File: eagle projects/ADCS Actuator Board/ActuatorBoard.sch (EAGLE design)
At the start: 281 parts, among them J19 TE_1-84953-1, J20 TE_1-84953-1, J21 TE_1-84953-1, U1 TVS991, U10 DRV10970_MOTOR_DRIVERDRV10970, U12 DRV10970_MOTOR_DRIVERDRV10970, U13 ADS7841E_2K5, U15 TLV9051IDCKR, U19 TLV9051IDCKR, U2 ADS7841E_2K5, U21 TLV9051IDCKR, U23 TLV9051IDCKR, U24 TLV9051IDCKR, U25 ADS7841E_2K5, U26 TLV9051IDCKR, U27 ADS7841E_2K5, U28 TLV9051IDCKR, U29 TLV9051IDCKR, U3 ADS7841E_2K5, U30 TLV9051IDCKR, U31 TLV9051IDCKR, U32 TLV9051IDCKR, U35 BD6210F-E2, U39 BD6210F-E2, U4 ADS7841E_2K5, U5 TVS991, U6 TLV9051IDCKR, U7 DRV10970_MOTOR_DRIVERDRV10970, U8 TVS991, U9 BD6210F-E2

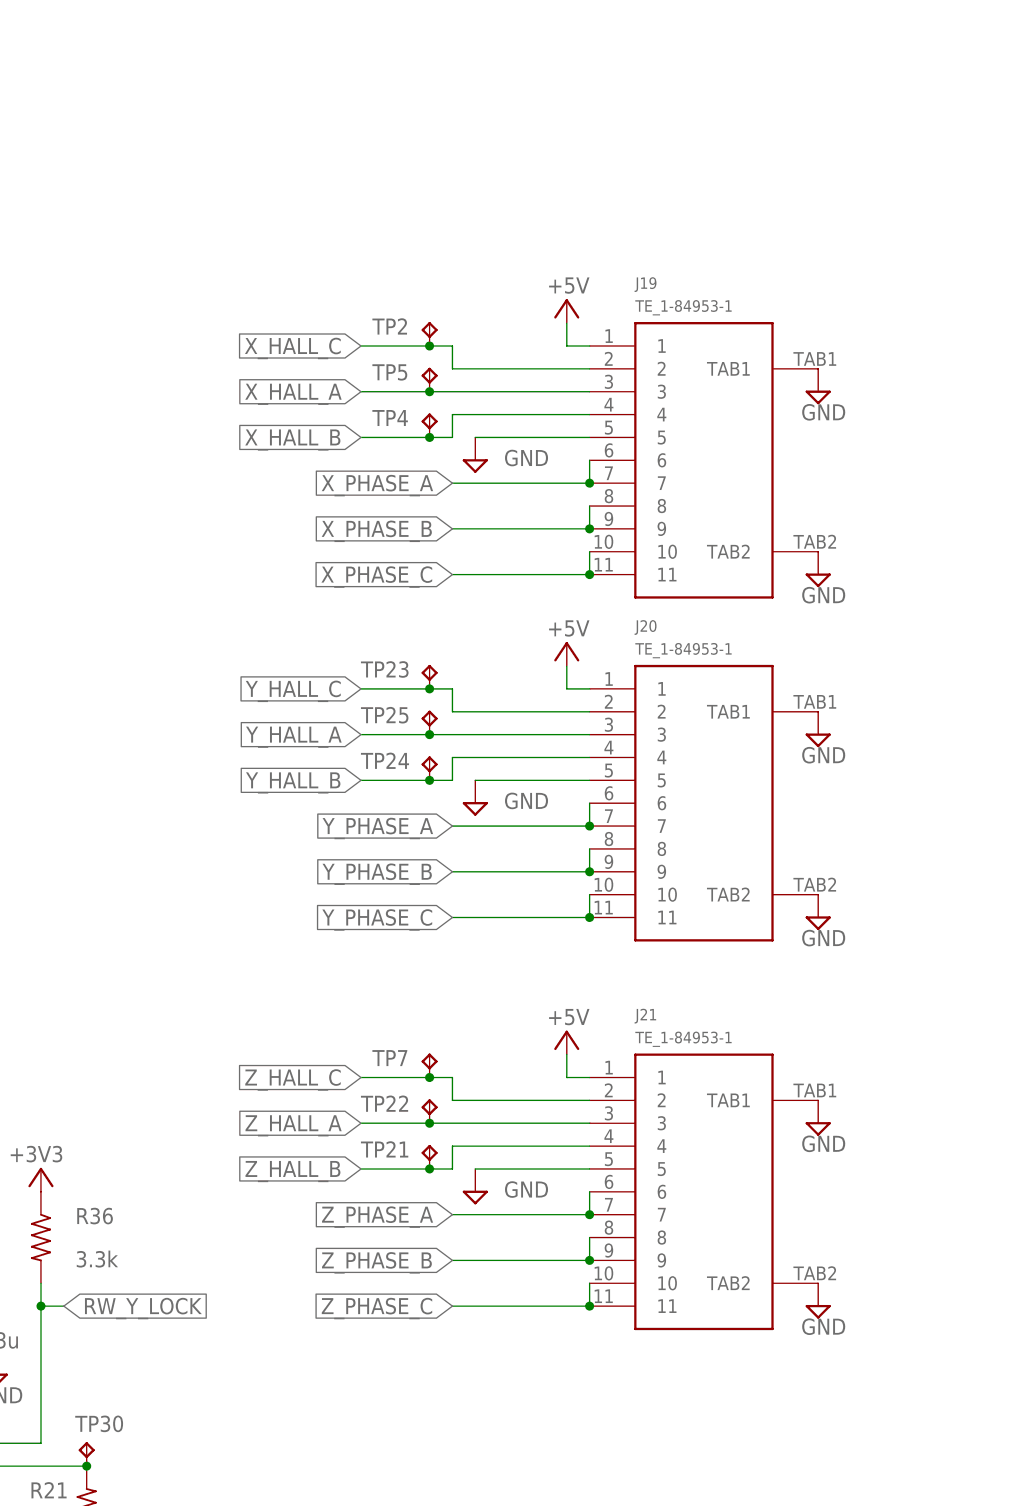
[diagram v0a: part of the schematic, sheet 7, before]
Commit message: DONE THIS MFER
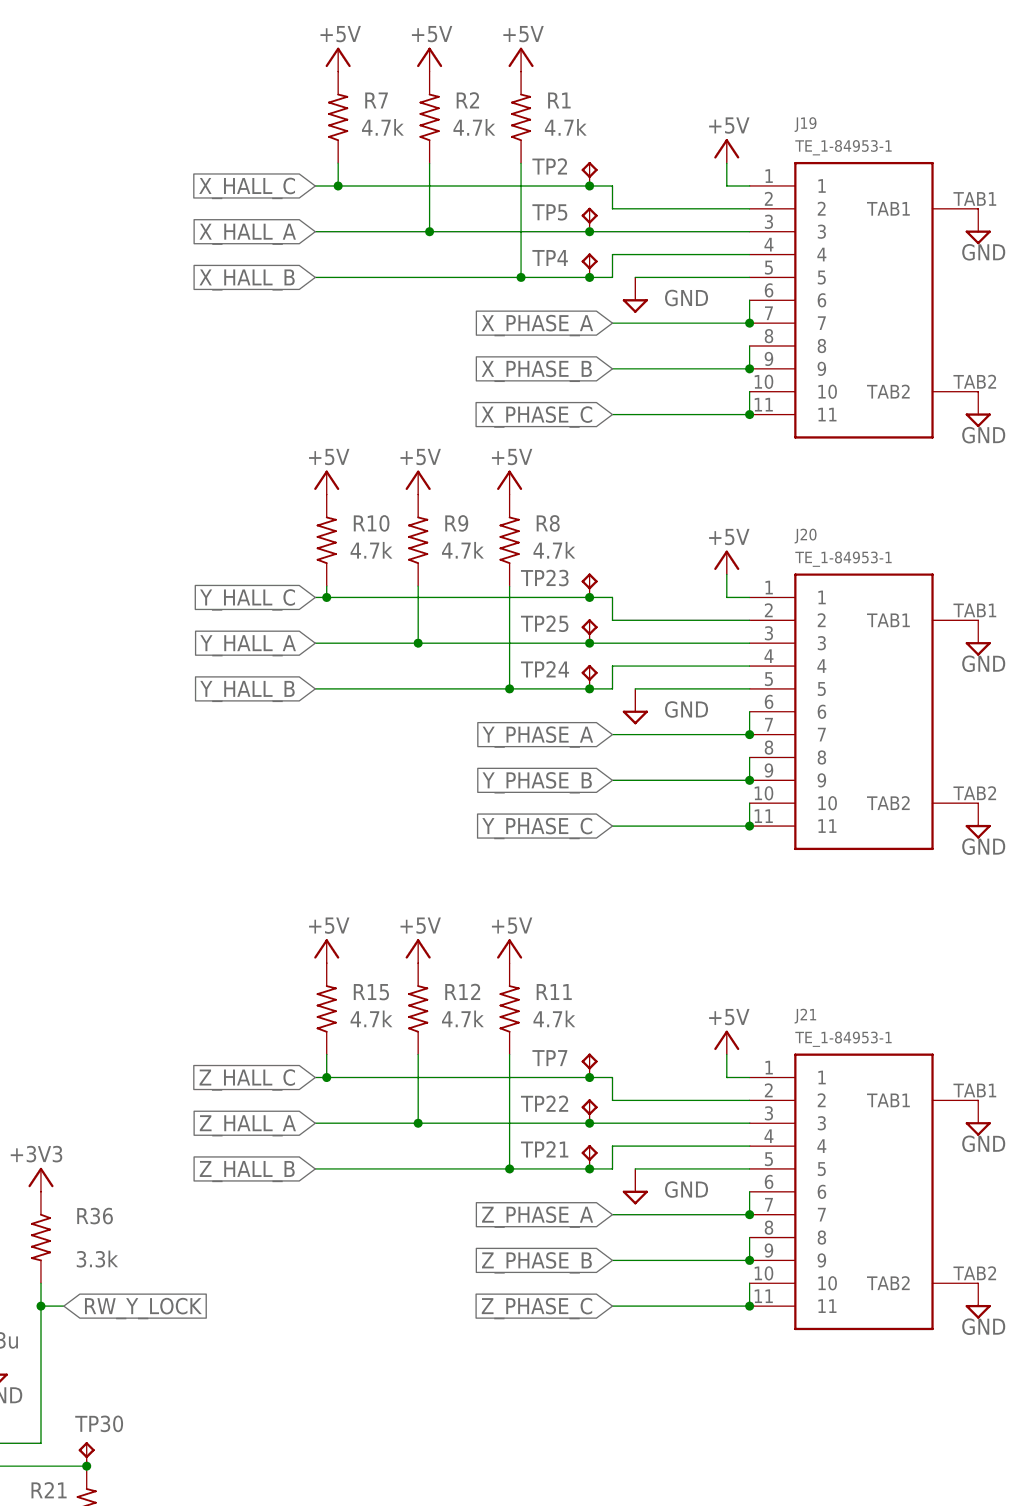
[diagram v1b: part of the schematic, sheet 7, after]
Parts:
- added R1, R10, R11, R12, R15, R2, R7, R8, R9: 4.7k, rcl:R-US_R0402
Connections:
- net +5V: now also R1.2, R10.2, R11.2, R12.2, R15.2, R2.2, R7.2, R8.2, R9.2
- net X_HALL_A: now also R2.1
- net X_HALL_B: now also R1.1
- net X_HALL_C: now also R7.1
- net Y_HALL_A: now also R9.1
- net Y_HALL_B: now also R8.1
- net Y_HALL_C: now also R10.1
- net Z_HALL_A: now also R12.1
- net Z_HALL_B: now also R11.1
- net Z_HALL_C: now also R15.1
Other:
- moved on the sheet: J19, J20, J21, TP2, TP21, TP22, TP23, TP24, TP25, TP4, TP5, TP7
